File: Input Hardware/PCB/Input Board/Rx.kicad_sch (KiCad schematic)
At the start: 32 parts

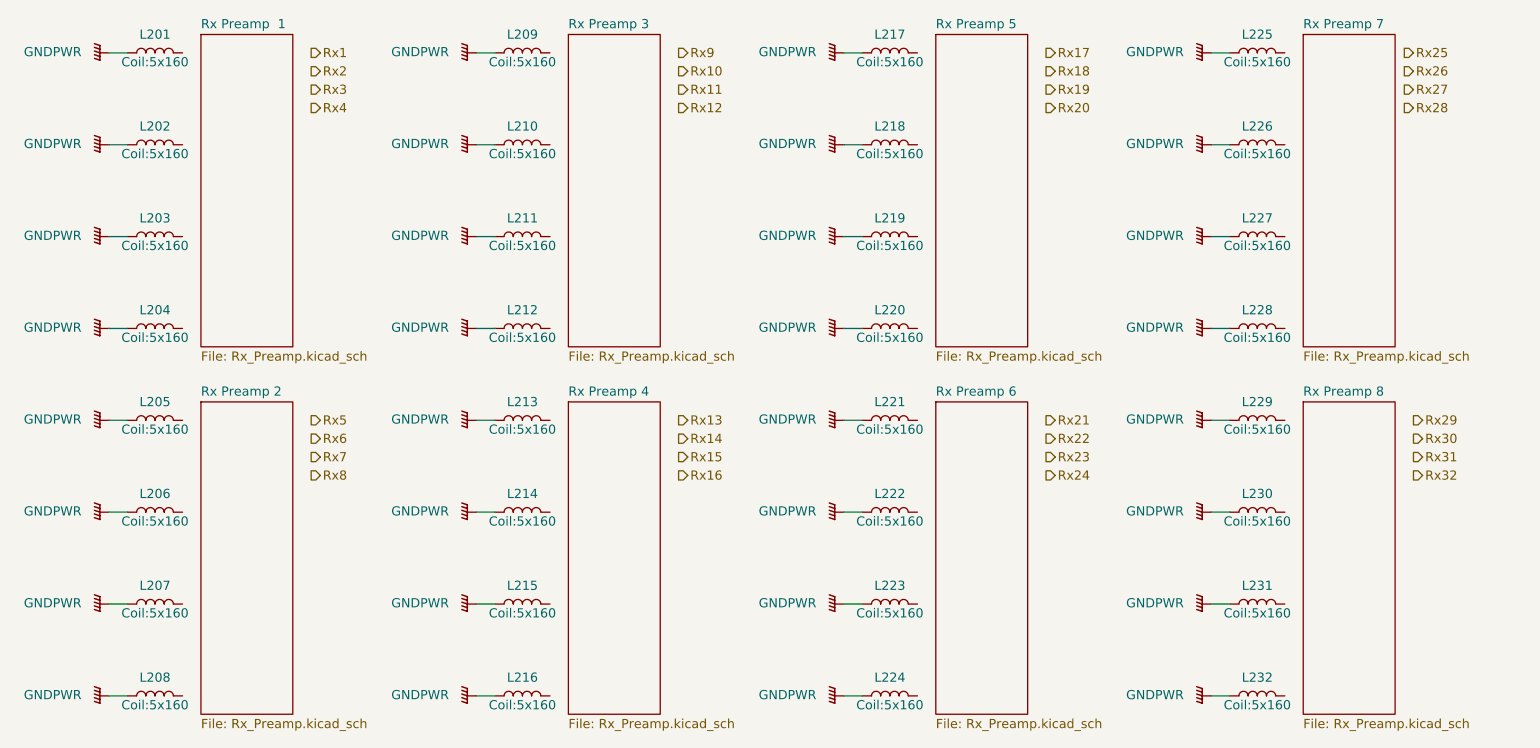
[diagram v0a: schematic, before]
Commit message: Update Schematic
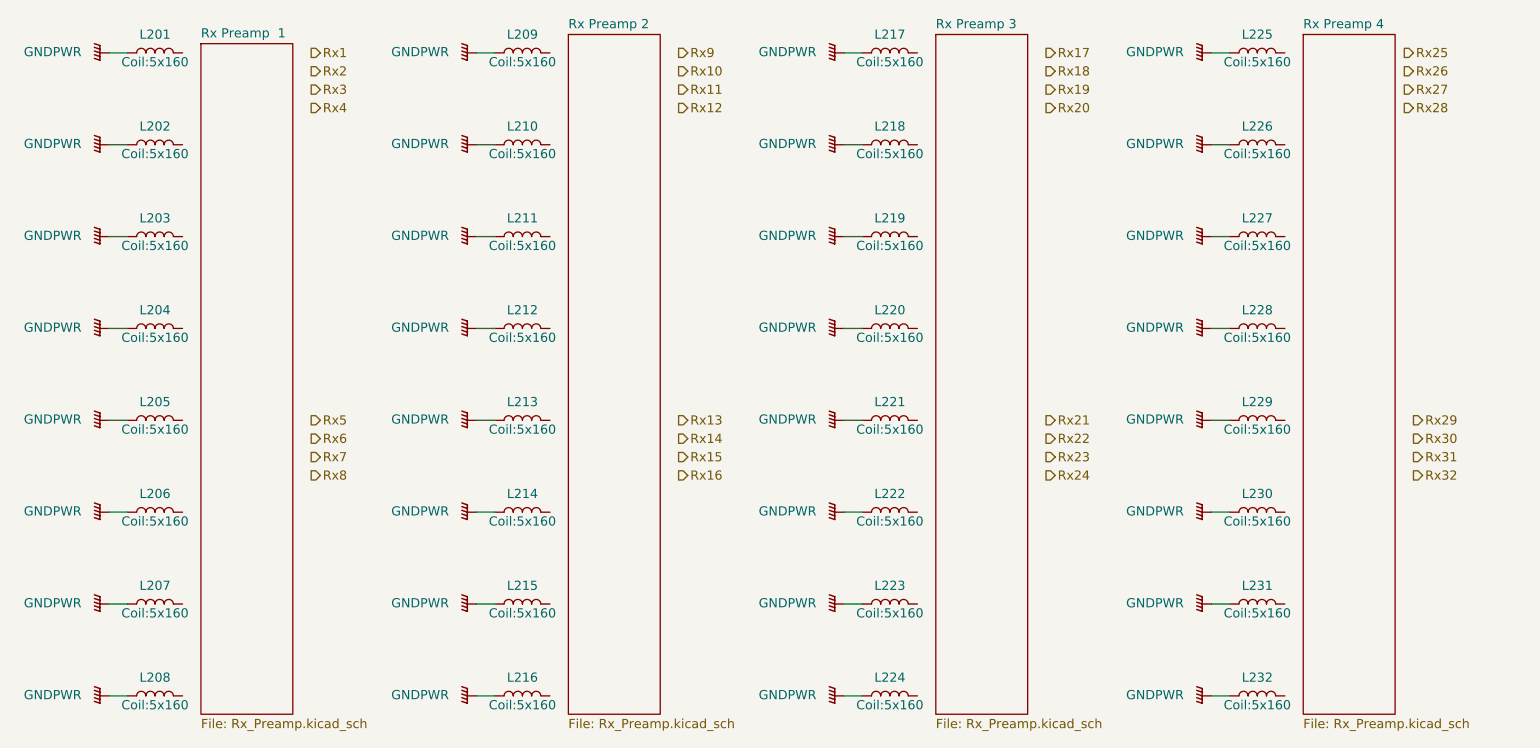
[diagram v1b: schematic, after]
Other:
- removed sheet Rx Preamp 5
- removed sheet Rx Preamp 6
- removed sheet Rx Preamp 7
- removed sheet Rx Preamp 8
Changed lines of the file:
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@@
 	)
 	(sheet
-		(at 101.6 73.66)
-		(size 12.7 43.18)
+		(at 203.2 22.86)
+		(size 12.7 93.98)
 		(exclude_from_sim no)
 		(in_bom yes)
@@
 		)
 		(property "Sheetname" "Rx Preamp 4"
-			(at 101.6 72.9484 0)
+			(at 203.2 22.1484 0)
+			(effects
+				(font
+					(size 1.27 1.27)
+				)
+				(justify left bottom)
+			)
+		)
+		(property "Sheetfile" "Rx_Preamp.kicad_sch"
+			(at 203.2 117.4246 0)
+			(effects
+				(font
+					(size 1.27 1.27)
+				)
+				(justify left top)
+			)
+		)
+		(instances
+			(project "Input Board"
+				(path "/198ad8d1-66e3-4deb-889c-1af2b81e67c3/e110e9b7-e557-4981-bab6-c28116ad040e"
+					(page "9")
+				)
+			)
+		)
+	)
+	(sheet
+		(at 152.4 22.86)
+		(size 12.7 93.98)
+		(exclude_from_sim no)
+		(in_bom yes)
+		(on_board yes)
+		(dnp no)
+		(fields_autoplaced yes)
+		(stroke
+			(width 0.1524)
+			(type solid)
+		)
+		(fill
+			(color 0 0 0 0.0000)
+		)
+		(property "Sheetname" "Rx Preamp 3"
+			(at 152.4 22.1484 0)
+			(effects
+				(font
+					(size 1.27 1.27)
+				)
+				(justify left bottom)
+			)
+		)
+		(property "Sheetfile" "Rx_Preamp.kicad_sch"
+			(at 152.4 117.4246 0)
+			(effects
+				(font
+					(size 1.27 1.27)
+				)
+				(justify left top)
+			)
+		)
+		(instances
+			(project "Input Board"
+				(path "/198ad8d1-66e3-4deb-889c-1af2b81e67c3/e110e9b7-e557-4981-bab6-c28116ad040e"
+					(page "7")
+				)
+			)
+		)
+	)
+	(sheet
+		(at 101.6 22.86)
+		(size 12.7 93.98)
+		(exclude_from_sim no)
+		(in_bom yes)
+		(on_board yes)
+		(dnp no)
+		(fields_autoplaced yes)
+		(stroke
+			(width 0.1524)
+			(type solid)
+		)
+		(fill
+			(color 0 0 0 0.0000)
+		)
+		(property "Sheetname" "Rx Preamp 2"
+			(at 101.6 22.1484 0)
 			(effects
 				(font
@@
 			(project "Input Board"
 				(path "/198ad8d1-66e3-4deb-889c-1af2b81e67c3/e110e9b7-e557-4981-bab6-c28116ad040e"
-					(page "6")
-				)
-			)
-		)
-	)
-	(sheet
-		(at 203.2 22.86)
-		(size 12.7 43.18)
-		(exclude_from_sim no)
-		(in_bom yes)
-		(on_board yes)
-		(dnp no)
-		(fields_autoplaced yes)
-		(stroke
-			(width 0.1524)
-			(type solid)
-		)
-		(fill
-			(color 0 0 0 0.0000)
-		)
-		(property "Sheetname" "Rx Preamp 7"
-			(at 203.2 22.1484 0)
-			(effects
-				(font
-					(size 1.27 1.27)
-				)
-				(justify left bottom)
-			)
-		)
-		(property "Sheetfile" "Rx_Preamp.kicad_sch"
-			(at 203.2 66.6246 0)
-			(effects
-				(font
-					(size 1.27 1.27)
-				)
-				(justify left top)
-			)
-		)
-		(instances
-			(project "Input Board"
-				(path "/198ad8d1-66e3-4deb-889c-1af2b81e67c3/e110e9b7-e557-4981-bab6-c28116ad040e"
-					(page "9")
-				)
-			)
-		)
-	)
-	(sheet
-		(at 152.4 22.86)
-		(size 12.7 43.18)
-		(exclude_from_sim no)
-		(in_bom yes)
-		(on_board yes)
-		(dnp no)
-		(fields_autoplaced yes)
-		(stroke
-			(width 0.1524)
-			(type solid)
-		)
-		(fill
-			(color 0 0 0 0.0000)
-		)
-		(property "Sheetname" "Rx Preamp 5"
-			(at 152.4 22.1484 0)
-			(effects
-				(font
-					(size 1.27 1.27)
-				)
-				(justify left bottom)
-			)
-		)
-		(property "Sheetfile" "Rx_Preamp.kicad_sch"
-			(at 152.4 66.6246 0)
-			(effects
-				(font
-					(size 1.27 1.27)
-				)
-				(justify left top)
-			)
-		)
-		(instances
-			(project "Input Board"
-				(path "/198ad8d1-66e3-4deb-889c-1af2b81e67c3/e110e9b7-e557-4981-bab6-c28116ad040e"
-					(page "7")
-				)
-			)
-		)
-	)
-	(sheet
-		(at 101.6 22.86)
-		(size 12.7 43.18)
-		(exclude_from_sim no)
-		(in_bom yes)
-		(on_board yes)
-		(dnp no)
-		(fields_autoplaced yes)
-		(stroke
-			(width 0.1524)
-			(type solid)
-		)
-		(fill
-			(color 0 0 0 0.0000)
-		)
-		(property "Sheetname" "Rx Preamp 3"
-			(at 101.6 22.1484 0)
-			(effects
-				(font
-					(size 1.27 1.27)
-				)
-				(justify left bottom)
-			)
-		)
-		(property "Sheetfile" "Rx_Preamp.kicad_sch"
-			(at 101.6 66.6246 0)
-			(effects
-				(font
-					(size 1.27 1.27)
-				)
-				(justify left top)
-			)
-		)
-		(instances
-			(project "Input Board"
-				(path "/198ad8d1-66e3-4deb-889c-1af2b81e67c3/e110e9b7-e557-4981-bab6-c28116ad040e"
 					(page "5")
 				)
@@
 	)
 	(sheet
-		(at 203.2 73.66)
-		(size 12.7 43.18)
-		(exclude_from_sim no)
-		(in_bom yes)
-		(on_board yes)
-		(dnp no)
-		(fields_autoplaced yes)
-		(stroke
-			(width 0.1524)
-			(type solid)
-		)
-		(fill
-			(color 0 0 0 0.0000)
-		)
-		(property "Sheetname" "Rx Preamp 8"
-			(at 203.2 72.9484 0)
-			(effects
-				(font
-					(size 1.27 1.27)
-				)
-				(justify left bottom)
-			)
-		)
-		(property "Sheetfile" "Rx_Preamp.kicad_sch"
-			(at 203.2 117.4246 0)
-			(effects
-				(font
-					(size 1.27 1.27)
-				)
-				(justify left top)
-			)
-		)
-		(instances
-			(project "Input Board"
-				(path "/198ad8d1-66e3-4deb-889c-1af2b81e67c3/e110e9b7-e557-4981-bab6-c28116ad040e"
-					(page "10")
-				)
-			)
-		)
-	)
-	(sheet
-		(at 50.8 73.66)
-		(size 12.7 43.18)
-		(exclude_from_sim no)
-		(in_bom yes)
-		(on_board yes)
-		(dnp no)
-		(fields_autoplaced yes)
-		(stroke
-			(width 0.1524)
-			(type solid)
-		)
-		(fill
-			(color 0 0 0 0.0000)
-		)
-		(property "Sheetname" "Rx Preamp 2"
-			(at 50.8 72.9484 0)
-			(effects
-				(font
-					(size 1.27 1.27)
-				)
-				(justify left bottom)
-			)
-		)
-		(property "Sheetfile" "Rx_Preamp.kicad_sch"
-			(at 50.8 117.4246 0)
-			(effects
-				(font
-					(size 1.27 1.27)
-				)
-				(justify left top)
-			)
-		)
-		(instances
-			(project "Input Board"
-				(path "/198ad8d1-66e3-4deb-889c-1af2b81e67c3/e110e9b7-e557-4981-bab6-c28116ad040e"
-					(page "4")
-				)
-			)
-		)
-	)
-	(sheet
-		(at 152.4 73.66)
-		(size 12.7 43.18)
-		(exclude_from_sim no)
-		(in_bom yes)
-		(on_board yes)
-		(dnp no)
-		(fields_autoplaced yes)
-		(stroke
-			(width 0.1524)
-			(type solid)
-		)
-		(fill
-			(color 0 0 0 0.0000)
-		)
-		(property "Sheetname" "Rx Preamp 6"
-			(at 152.4 72.9484 0)
-			(effects
-				(font
-					(size 1.27 1.27)
-				)
-				(justify left bottom)
-			)
-		)
-		(property "Sheetfile" "Rx_Preamp.kicad_sch"
-			(at 152.4 117.4246 0)
-			(effects
-				(font
-					(size 1.27 1.27)
-				)
-				(justify left top)
-			)
-		)
-		(instances
-			(project "Input Board"
-				(path "/198ad8d1-66e3-4deb-889c-1af2b81e67c3/e110e9b7-e557-4981-bab6-c28116ad040e"
-					(page "8")
-				)
-			)
-		)
-	)
-	(sheet
-		(at 50.8 22.86)
-		(size 12.7 43.18)
+		(at 50.8 24.13)
+		(size 12.7 92.71)
 		(exclude_from_sim no)
 		(in_bom yes)
@@
 		)
 		(property "Sheetname" "Rx Preamp  1"
-			(at 50.8 22.1484 0)
+			(at 50.8 23.4184 0)
 			(effects
 				(font
@@
 		)
 		(property "Sheetfile" "Rx_Preamp.kicad_sch"
-			(at 50.8 66.6246 0)
+			(at 50.8 117.4246 0)
 			(effects
 				(font

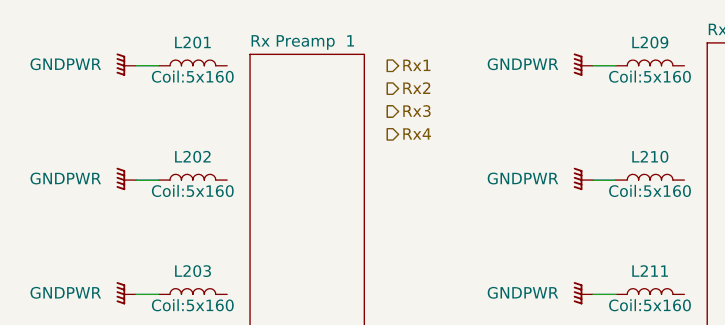
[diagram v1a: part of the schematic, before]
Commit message: Fix Name
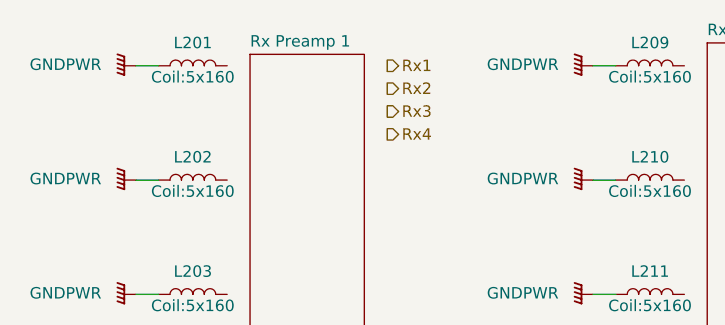
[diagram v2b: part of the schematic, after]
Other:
- sheet Rx Preamp  1 renamed Rx Preamp 1
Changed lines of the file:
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@@
 			(color 0 0 0 0.0000)
 		)
-		(property "Sheetname" "Rx Preamp  1"
+		(property "Sheetname" "Rx Preamp 1"
 			(at 50.8 23.4184 0)
 			(effects
